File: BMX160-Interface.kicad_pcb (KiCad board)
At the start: 2 copper layers, 5.4 x 3.9 mm, 2 parts, among them U1 BMX160, U2 BNO085

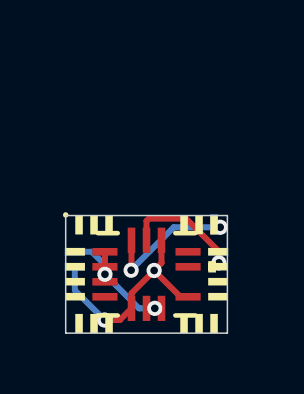
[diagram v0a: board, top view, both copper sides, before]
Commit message: Updated board
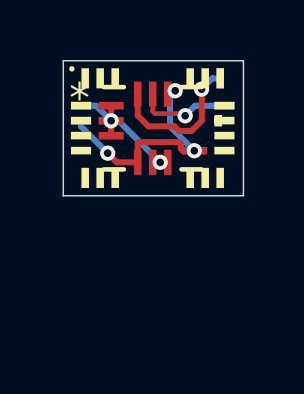
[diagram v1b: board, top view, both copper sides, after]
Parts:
- moved U1 4.87 mm to (130.0, 82.0)
- moved U2 4.87 mm to (130.0, 82.0)
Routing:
- net /SCL: track 4.30 -> 3.16 mm
- net +3V3: track 7.42 -> 8.01 mm, vias 2 -> 3
- net /SDA: track 4.82 -> 5.03 mm, vias 2 -> 1
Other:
- board size 5.4 x 3.9 mm -> 6 x 4.5 mm
